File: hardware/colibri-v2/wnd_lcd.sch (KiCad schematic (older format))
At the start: 18 parts

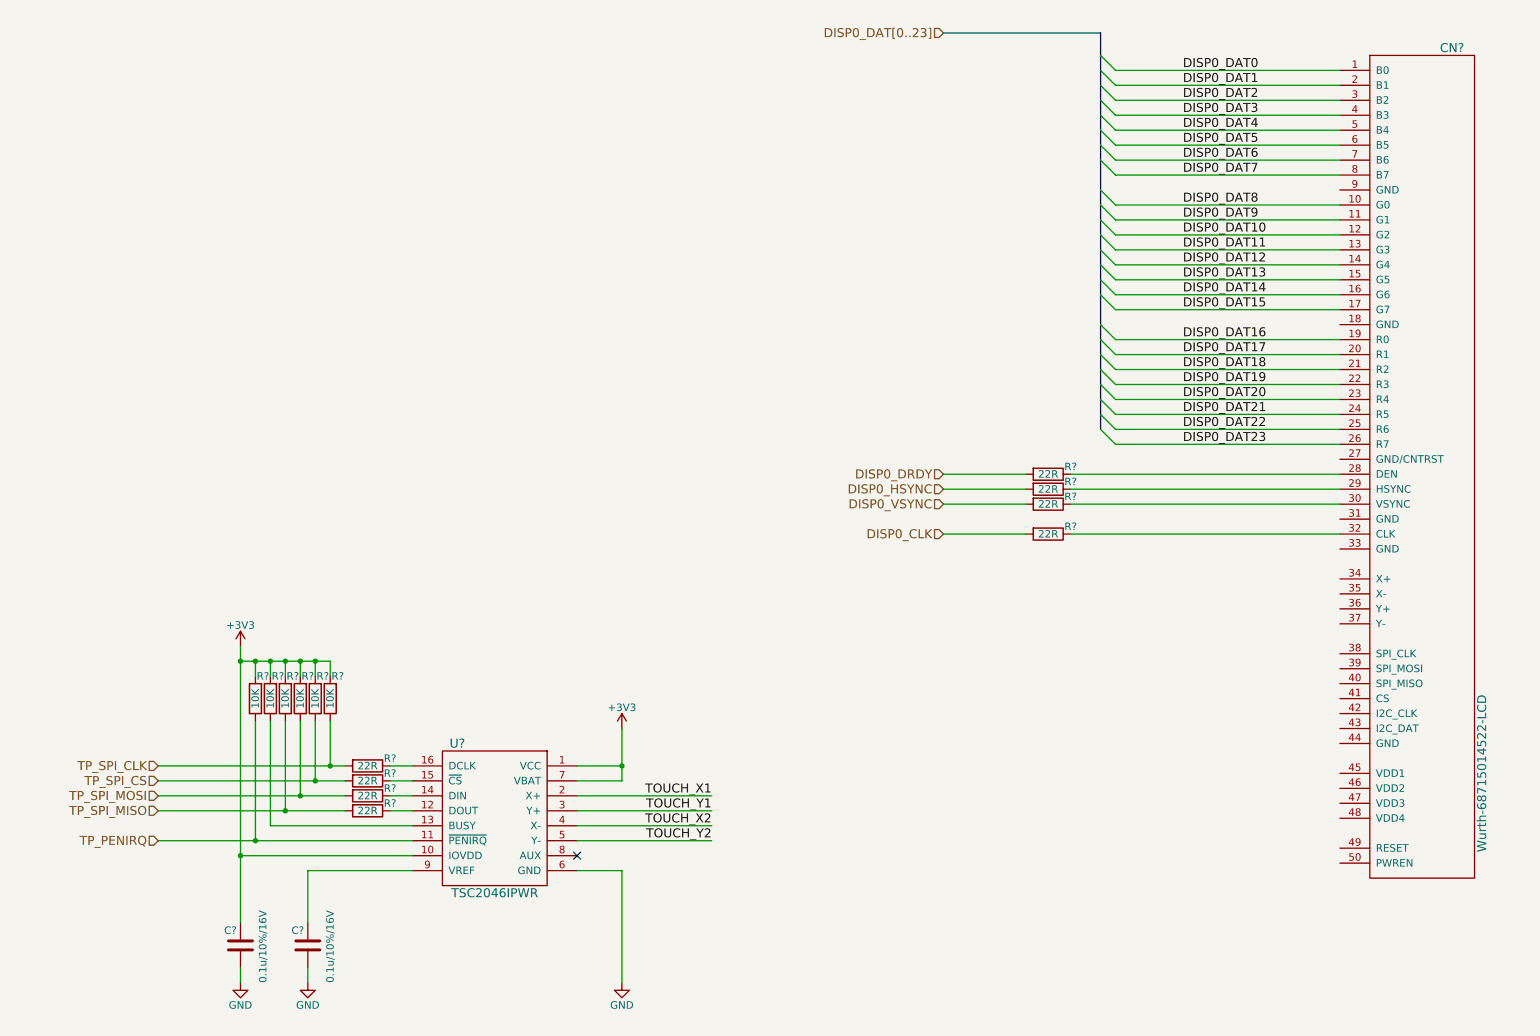
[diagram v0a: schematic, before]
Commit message: Work on Wandboard LCD
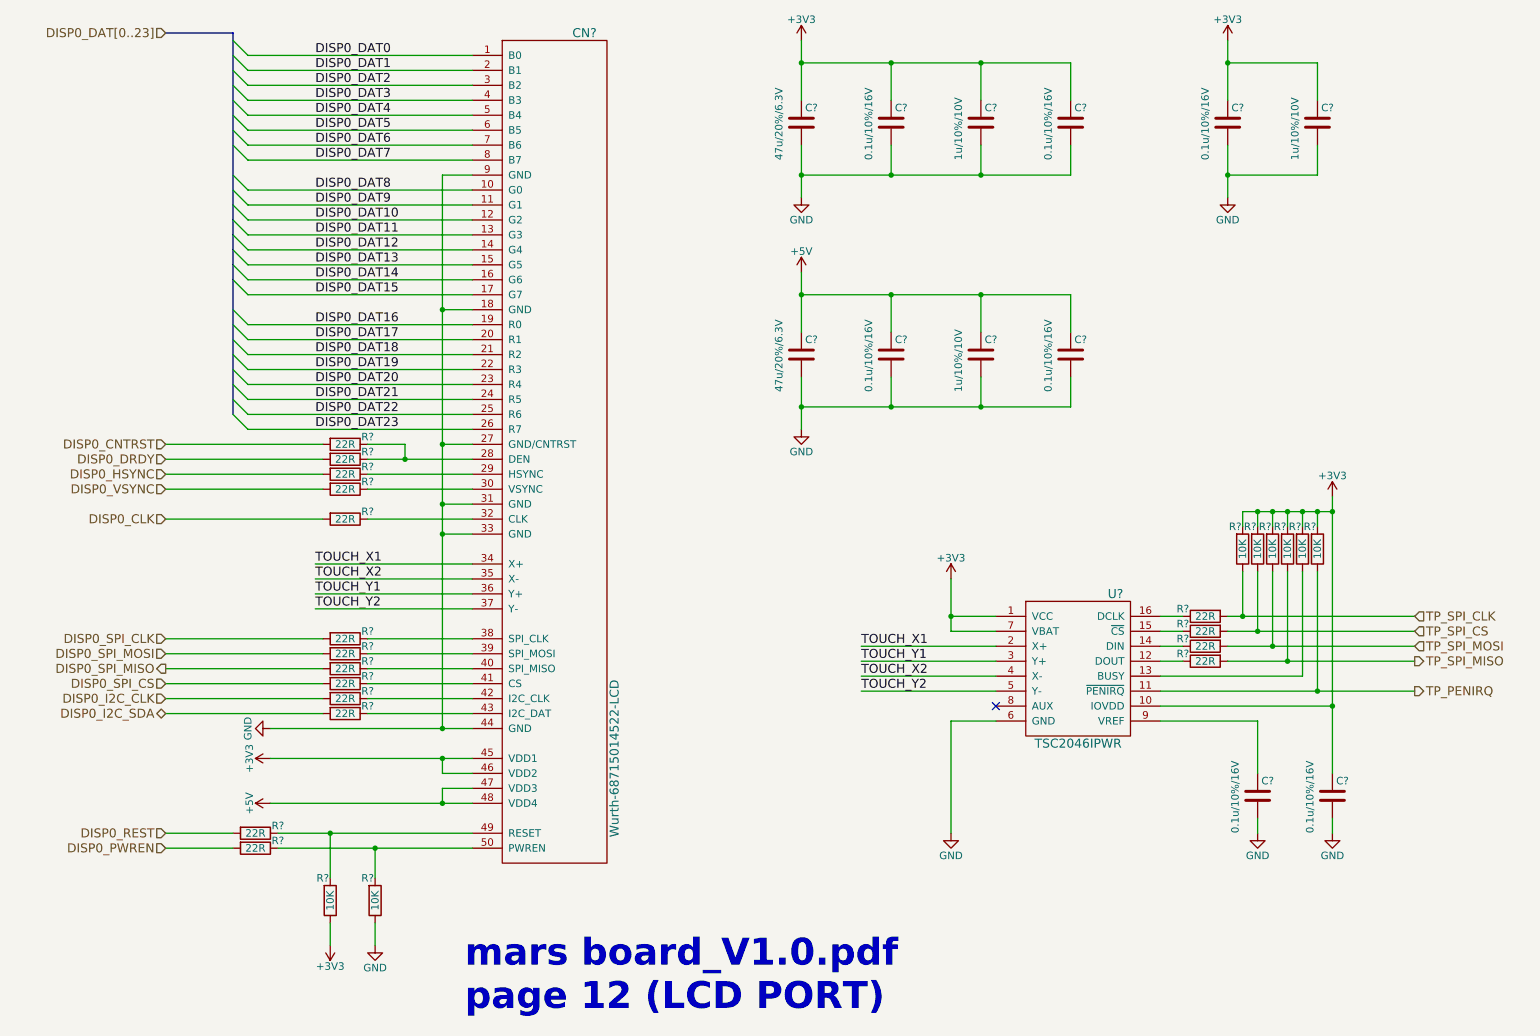
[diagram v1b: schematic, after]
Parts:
- added C? (x3): 1u/10%/10V, symbol C
- added C? (x2): 47u/20%/6.3V, symbol C
- added C? (x5): 0.1u/10%/16V, symbol C
- added R? (x9): 22R, symbol R
- added R? (x2): 10K, symbol R
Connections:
- net +3V3: now also CN?.45 (VDD1), CN?.46 (VDD2), C?.1, C?.1, C?.1, C?.1, C?.1, C?.1, R?.1
- net GND: now also CN?.18 (GND), CN?.27 (GND/CNTRST), CN?.31 (GND), CN?.33 (GND), CN?.44 (GND), CN?.9 (GND), C?.2, C?.2, C?.2, C?.2, C?.2, C?.2, C?.2, C?.2, C?.2, C?.2, R?.1
- net TOUCH_X1: now also CN?.34 (X+)
- net TOUCH_X2: now also CN?.35 (X-)
- net TOUCH_Y1: now also CN?.36 (Y+)
- net TOUCH_Y2: now also CN?.37 (Y-)
- net at CN?.28 (DEN), R?.1: now also R?.1
- net at CN?.38 (SPI_CLK): now also R?.1
- net at CN?.39 (SPI_MOSI): now also R?.1
- net at CN?.40 (SPI_MISO): now also R?.1
- net at CN?.41 (CS): now also R?.1
- net at CN?.42 (I2C_CLK): now also R?.1
- net at CN?.43 (I2C_DAT): now also R?.1
- net +5V: now reaches CN?.47 (VDD3)
- net +5V: now also CN?.48 (VDD4), C?.1, C?.1, C?.1, C?.1
- net at CN?.49 (RESET): now also R?.1, R?.2
- net at CN?.50 (PWREN): now also R?.1, R?.2
- new net DISP0_CNTRST: R?.2
- new net DISP0_I2C_CLK: R?.2
- new net DISP0_I2C_SDA: R?.2
- new net DISP0_PWREN: R?.2
- new net DISP0_REST: R?.2
- new net DISP0_SPI_CLK: R?.2
- new net DISP0_SPI_CS: R?.2
- new net DISP0_SPI_MISO: R?.2
- new net DISP0_SPI_MOSI: R?.2
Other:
- note added: "mars board_V1.0.pdf\npage 12 (LCD PORT)"
- moved on the sheet: C?, CN?, R?, U?
